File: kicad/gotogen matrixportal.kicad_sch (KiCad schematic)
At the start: 27 parts, among them J1 HUB75 Out, J2 HUB75 In, J3 OLED_128_64, J4 Buttons EXT, J5 OpenMV, J6 Extra Connections, J7 Capacitive Touch, SW1 Back, SW2 Menu, SW3 Up, SW4 Down, SW5 Extra1, SW6 Extra2, U1 MatrixPortal_M4, U2 PCF8523_Breakout, U3 PCF8574, U4 MPR121_Breakout, U5 MAX9814_Breakout

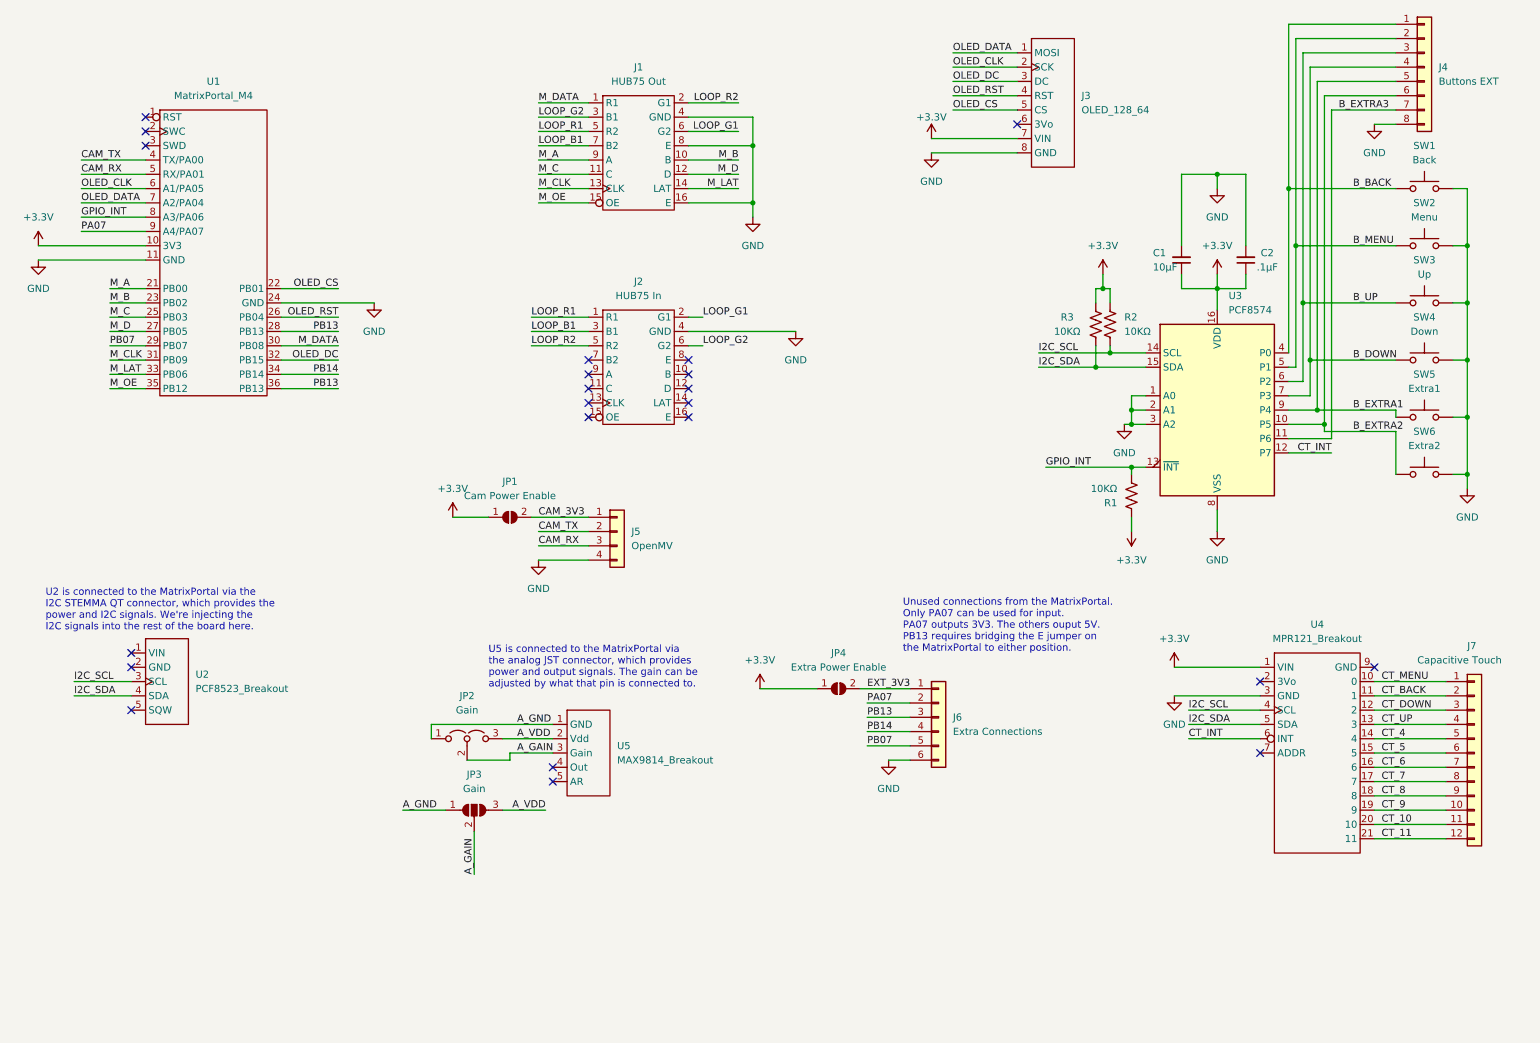
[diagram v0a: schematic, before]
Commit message: first pass at pcb update
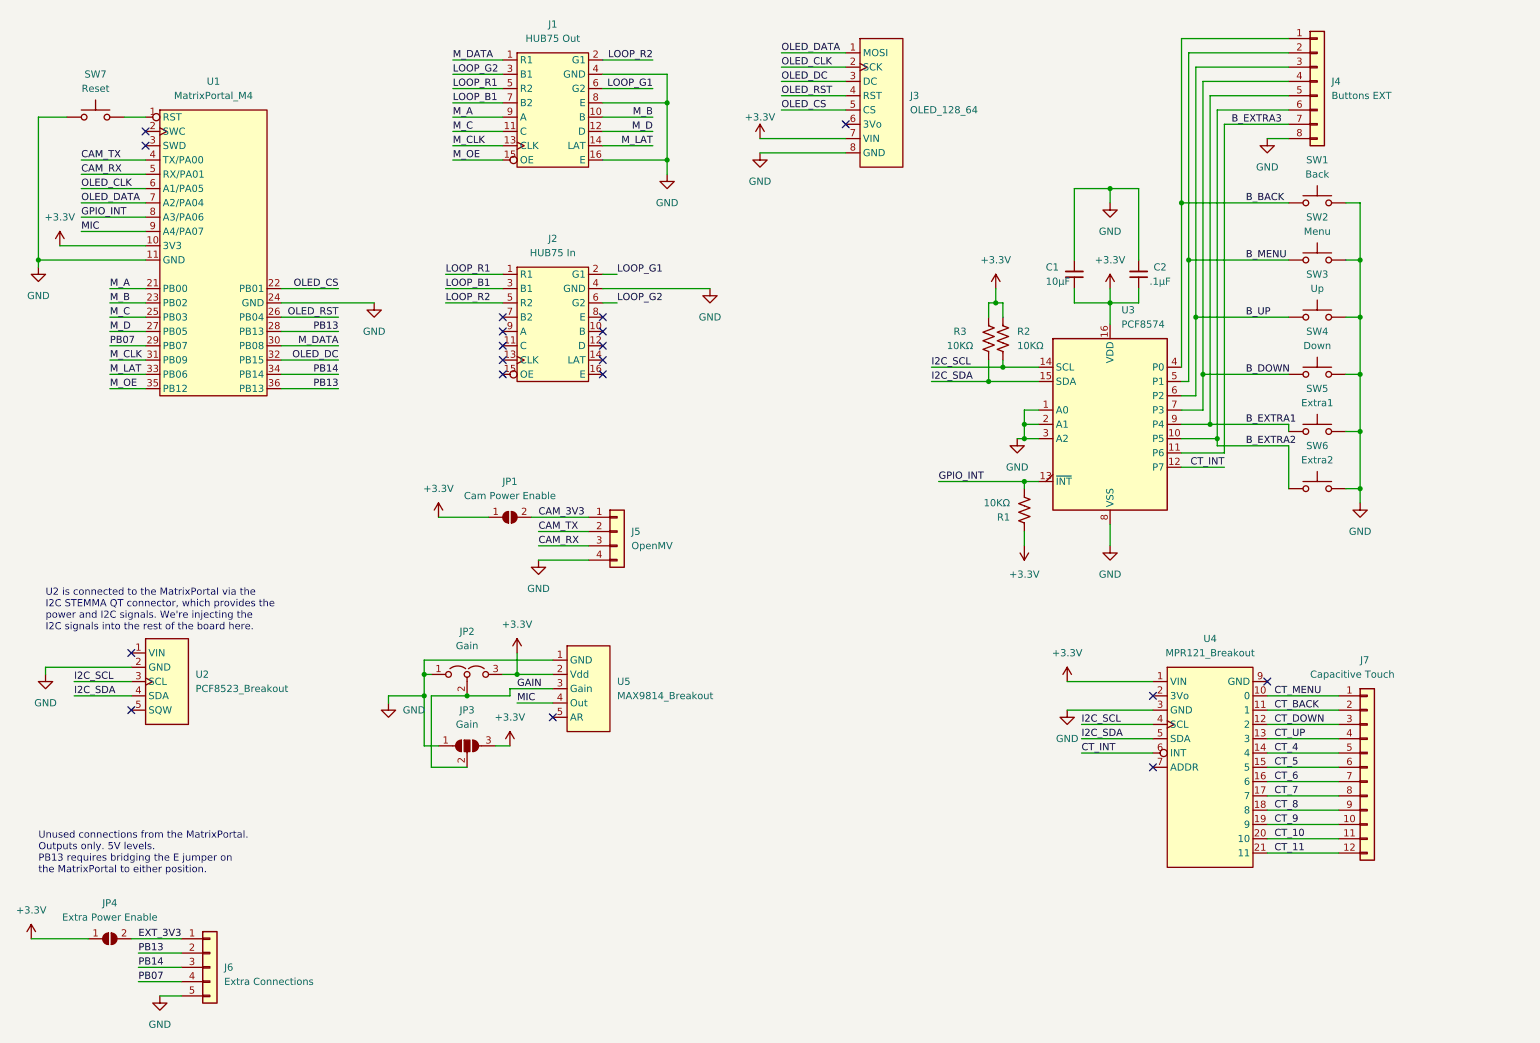
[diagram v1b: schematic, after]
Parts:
- added SW7: Reset, Button_Switch_THT:SW_PUSH_6mm, symbol Switch:SW_Push
- J6: footprint Connector_PinHeader_2.54mm:PinHeader_1x06_P2.54mm_Vertical -> Connector_PinHeader_2.54mm:PinHeader_1x05_P2.54mm_Vertical; symbol Connector_Generic:Conn_01x06 -> Connector_Generic:Conn_01x05
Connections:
- net A_GND is gone; now on net GND: JP2.1 (A), JP3.1 (A), U5.1 (GND)
- net A_VDD is gone; now on net +3.3V: JP2.3 (B), JP3.3 (B), U5.2 (Vdd)
- net GND: now also J6.5 (Pin_5), U2.2 (GND), SW7.1; no longer J6.6 (Pin_6)
- net PB07: now also J6.4 (Pin_4); no longer J6.5 (Pin_5)
- net PB13: now also J6.2 (Pin_2); no longer J6.3 (Pin_3)
- net PB14: now also J6.3 (Pin_3); no longer J6.4 (Pin_4)
- net at U1.1 (RST): now also SW7.2
- net MIC: now reaches U5.4 (Out)
- net MIC: now also U1.9 (A4/PA07)
- net A_GAIN renamed GAIN
- removed net PA07: J6.2 (Pin_2), U1.9 (A4/PA07)
- no-connect marks 22 -> 19
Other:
- note added: "Unused connections from the MatrixPortal. Outputs only. 5V levels. PB13 requires bridging the E jumper on the MatrixPortal to either position."
- note removed: "U5 is connected to the MatrixPortal via the analog JST connector, which provides power and output signals. The gain can be adjusted by what that pin is connected to."
- note removed: "Unused connections from the MatrixPortal. Only PA07 can be used for input. PA07 outputs 3V3. The others ouput 5V. PB13 requires bridging the E jumper on the MatrixPortal to either position."
- company: (none) -> Andy Janata
- title: (none) -> Gotogen Matrix Portal
- moved on the sheet: C1, C2, J4, J7, JP2, JP3, JP4, R1, R2, R3, SW1, SW2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
